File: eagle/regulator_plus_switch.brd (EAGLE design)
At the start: 184.7 x 181.9 mm, 43 parts, among them IC2 LT1352PA, IC3 DG419DJN, IC4 LT1352PA, J17 5669-8, J23 5569-2, J24 5569-2, J25 5569-2, J26 5569-2

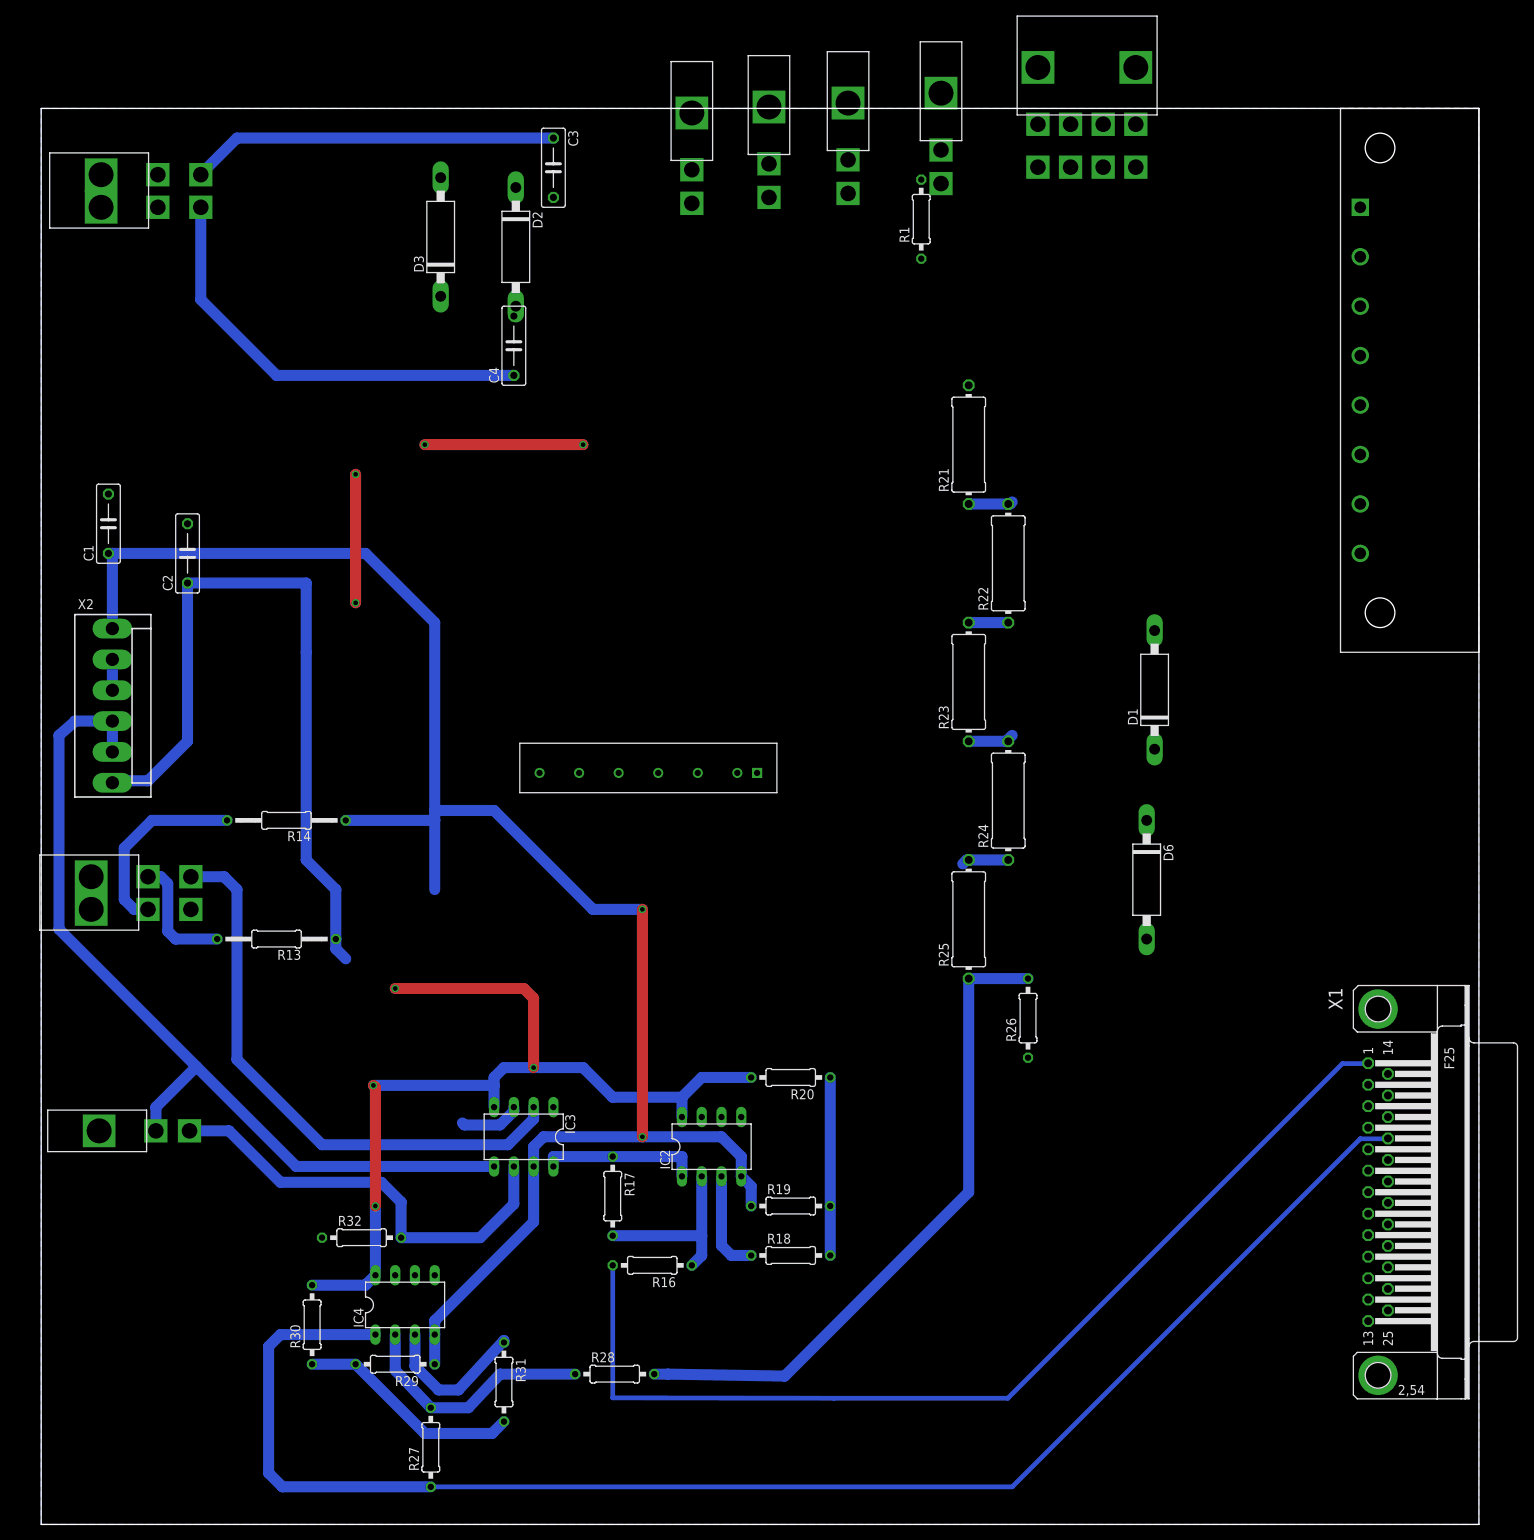
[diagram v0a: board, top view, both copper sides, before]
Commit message: Test layouts pa97
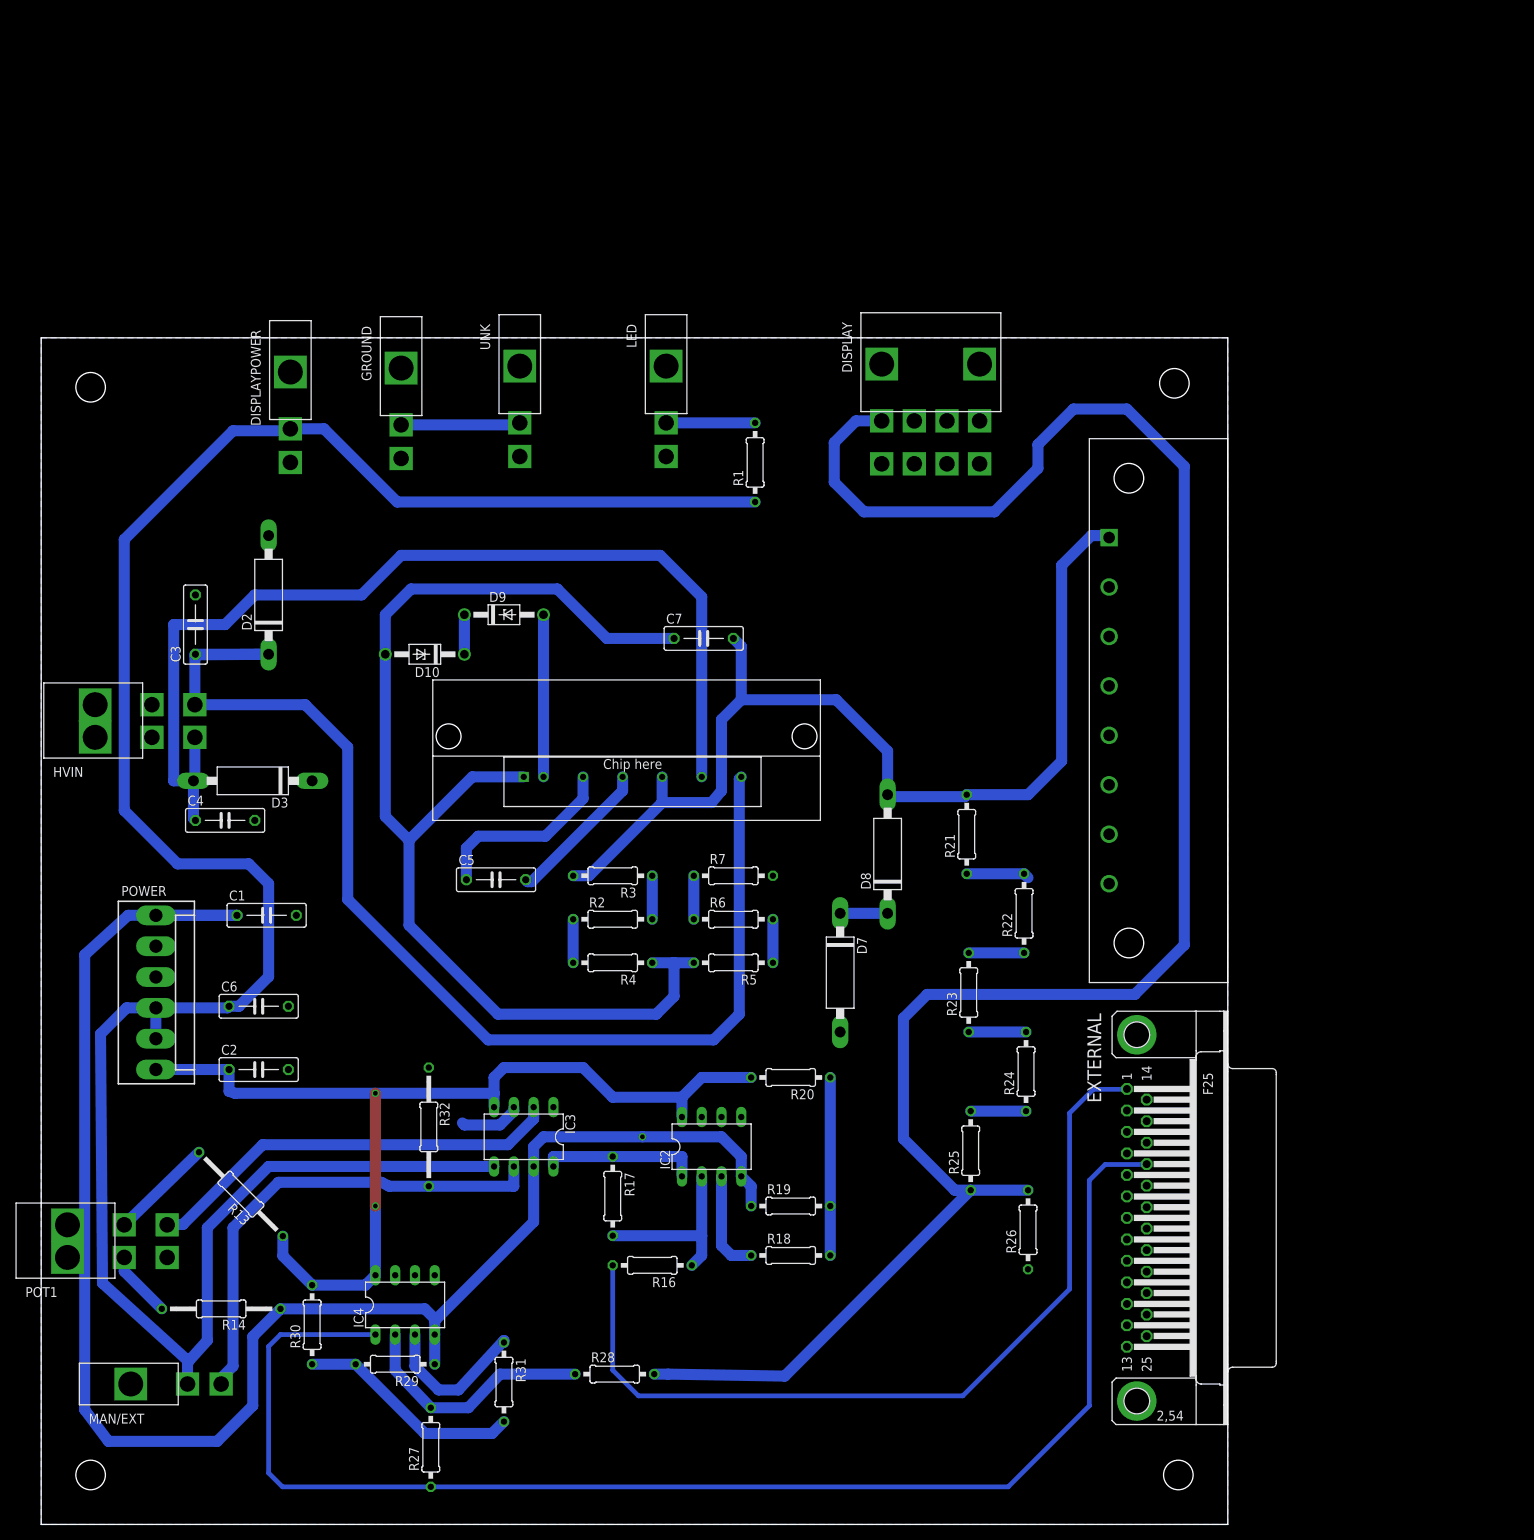
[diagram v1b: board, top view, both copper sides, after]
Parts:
- removed D1, D6: P6KEXXA, diode:C1702-15
- removed J17: 5669-8, con-molex:5669-8
- removed J23, J24, J25, J26: 5569-2, con-molex:5569-2
- removed U$1, U$2: 5569-4, con-molex:5669-4
- removed U$3: PA97, apex:7SIP
- removed U$5: 640584-1, con-amp-te:640584-1
- removed X1: (no value), con-subd:F25HP
- removed X2: (no value), con-molex:KK-156-6
- added C5, C7: 10p, rcl:C075-032X103
- added C6: 10n, rcl:C075-032X103
- added D10, D9: 1n4742, diode:DO41Z10
- added D7, D8: P6KEXXA, diode:C1702-15
- added DISPLAY: 5669-8, con-molex:5669-8
- added DISPLAYPOWER, GROUND, LED, MAN/EXT, UNK: 5569-2, con-molex:5569-2
- added EXTERNAL: (no value), con-subd:F25HP
- added HVIN, POT1: 5569-4, con-molex:5669-4
- added KK1: SK125/50C247, heatsink:C247-050
- added OUT: 640584-1, con-amp-te:640584-1
- added POWER: (no value), con-molex:KK-156-6
- added R2, R3, R4: 1M, rcl:0207/10
- added R5, R6, R7: 25.5k, rcl:0207/10
- R21, R22, R23, R24, R25: device resistor:0414/15 -> resistor:0207/10
- R26: value 50k -> 5k
- R32: device rcl:0207/10 -> rcl:0207/15
- U$4: value 5569-2 -> PA97; device con-molex:5569-2 -> apex:7SIP
- moved C3 74.5 mm to (19.8, 115.6), turned to 90 degrees
- moved D3 73.9 mm to (27.2, 95.5), turned to 180 degrees
- moved C4 71.4 mm to (23.6, 90.4), turned to 0 degrees
- moved C2 66.9 mm to (27.9, 58.4), turned to 0 degrees
- moved U$4 65.6 mm to (62.0, 96.0), turned to 0 degrees
- moved R14 63.3 mm to (23.1, 27.7)
- moved D2 54.8 mm to (29.2, 119.4), turned to 90 degrees
- moved C1 54.2 mm to (29.0, 78.2), turned to 0 degrees
- moved R21 50.0 mm to (118.9, 88.6)
- moved R22 45.0 mm to (126.2, 78.5)
- moved R23 39.9 mm to (119.1, 68.3)
- moved R1 37.8 mm to (91.7, 136.4)
- moved R24 34.9 mm to (126.5, 58.2)
- moved R13 33.1 mm to (25.7, 42.4), turned to 135 degrees
- moved R25 29.7 mm to (119.4, 48.0)
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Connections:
- removed net N$1: D1.C, D6.C
- removed net N$10: D1.A, R21.2, U$5.P$1
- new net N$11: C7.2, D8.A, OUT.P$1, R21.2, R3.2, U$4.P$5
- new net N$12: R2.1, R4.2
- new net N$14: R5.1, R6.2
- new net N$16: R6.1, R7.1
- new net N$18: R2.2, R3.1
- new net N$29: D10.C, D9.C
- new net N$3: C5.1, U$4.P$3
- new net N$38: C7.1, D10.A, R4.1, R5.2, U$4.P$1
- new net N$4: C5.2, U$4.P$4
- new net N$8: D7.C, D8.C
- net +15V: now also POWER.6; no longer X2.6
- net +5V: now also C6.1, DISPLAYPOWER.P$1, MAN/EXT.P$1, POWER.4, POWER.5; no longer J25.P$1, U$4.P$1, X2.4, X2.5
- net -15V: now also POWER.1; no longer X2.1
- net CMD1: now also EXTERNAL.1; no longer X1.1
- net GND: now also C6.2, D7.A, DISPLAYPOWER.P$2, EXTERNAL.10, EXTERNAL.12, EXTERNAL.14, EXTERNAL.16, EXTERNAL.2, EXTERNAL.25, EXTERNAL.4, EXTERNAL.6, EXTERNAL.8, GROUND.P$2, HVIN.P$1, HVIN.P$2, LED.P$2, POWER.2, POWER.3, R7.2, UNK.P$2; no longer D6.A, J23.P$2, J24.P$2, J25.P$2, J26.P$2, U$2.P$1, U$2.P$2, X1.10, X1.12, X1.14, X1.16, X1.2, X1.25, X1.4, X1.6, X1.8, X2.2, X2.3
- net MAN: now also MAN/EXT.P$2; no longer U$4.P$2
- net N$13: now also POT1.P$4; no longer U$1.P$4
- net N$15: now also POT1.P$1; no longer U$1.P$1
- net N$28: now also D9.A, U$4.P$2
- net N$34: now also DISPLAY.P$1; no longer J17.P$1
- net N$35: now also EXTERNAL.17; no longer X1.17
- net N$6: now also GROUND.P$1, UNK.P$1; no longer J23.P$1, J24.P$1
- net N$7: now also LED.P$1; no longer J26.P$1
- net N$9: now also POT1.P$2; no longer U$1.P$2
- net V+: now also HVIN.P$4, U$4.P$7; no longer U$2.P$4, U$3.P$7
- net V-: now also HVIN.P$3, U$4.P$6; no longer U$2.P$3, U$3.P$6
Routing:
- net +5V: track 115.3 -> 297.2 mm
- net N$34: track 85.2 -> 255.4 mm
- net N$38: track 0.00 -> 149.7 mm
- net N$11: track 0.00 -> 132.4 mm
- net V+: track 47.8 -> 156.4 mm
- net +15V: track 216.3 -> 128.7 mm, vias 4 -> 2
- net V-: track 56.1 -> 130.3 mm
- net GND: track 48.7 -> 7.95 mm, vias 4 -> 0
- net N$35: track 212.7 -> 178.2 mm
- net N$3: track 0.00 -> 24.5 mm
- net CMD1: track 131.9 -> 110.4 mm
- net N$28: track 0.00 -> 20.8 mm
- net N$13: track 74.0 -> 54.2 mm
- net N$4: track 0.00 -> 19.2 mm
- net N$15: track 24.9 -> 8.60 mm
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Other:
- board size 184.7 x 181.9 mm -> 152.4 x 152.4 mm
